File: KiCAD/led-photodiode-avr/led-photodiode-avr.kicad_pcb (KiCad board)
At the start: 4 copper layers, 68.6 x 80 mm, 62 parts, among them J1 Screw_Terminal_01x02, J2 Conn_02x08_Odd_Even, J3 ISP, J4 Conn_01x06_Pin, Q1 TTC1949, Q2 TTC1949, Q3 TTC1949, Q4 TTC1949, U1 REF3040AIDBZT, U10 AZ1117CH2-5.0, U2 AZ1117CH2-5.0, U3 OPA365xxD, U5 DDC112, U6 LTC1380, U7 ATmega328-A, U8 OPA365xxD, U9 LTC2631, Y1 CO_16MHZ

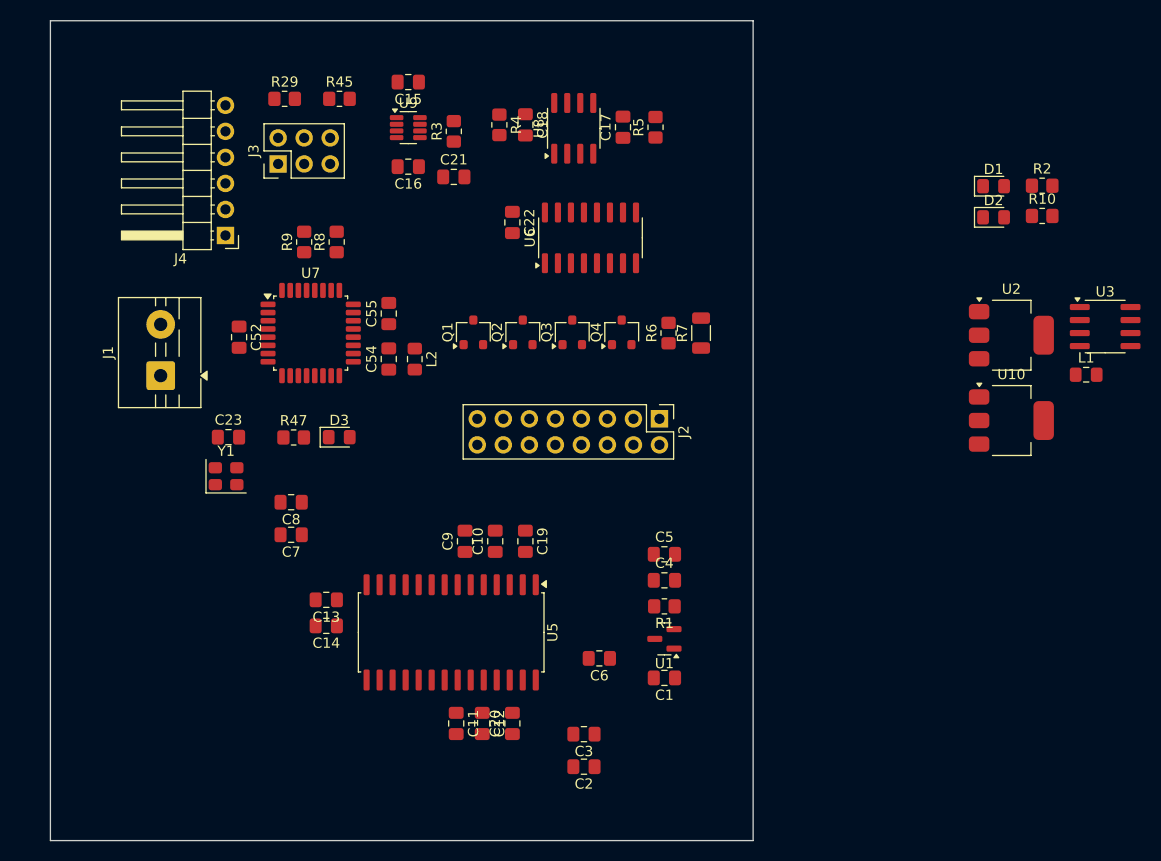
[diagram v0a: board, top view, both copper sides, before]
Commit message: routing done
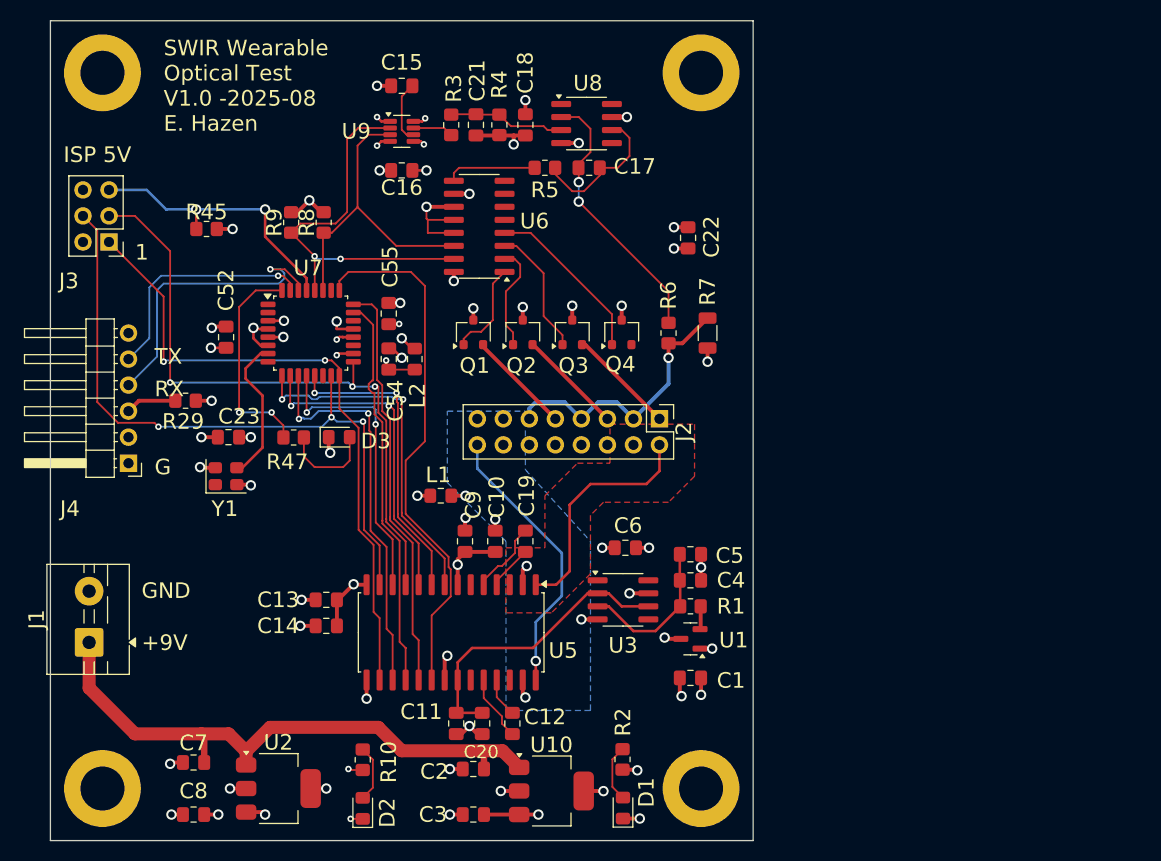
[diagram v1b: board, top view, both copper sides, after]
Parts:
- added H1: MountingHole, MountingHole:MountingHole_4.3mm_M4_DIN965_Pad, F.Cu at (121.9, 62.2)
- added H2: MountingHole, MountingHole:MountingHole_4.3mm_M4_DIN965_Pad, F.Cu at (180.3, 62.2)
- added H3: MountingHole, MountingHole:MountingHole_4.3mm_M4_DIN965_Pad, F.Cu at (121.9, 132.1)
- added H4: MountingHole, MountingHole:MountingHole_4.3mm_M4_DIN965_Pad, F.Cu at (180.3, 132.1)
- moved R10 84.9 mm to (147.3, 129.3), turned to 90 degrees
- moved D2 84.4 mm to (147.3, 134.0), turned to 90 degrees
- moved U2 84.1 mm to (139.1, 132.1)
- moved D1 70.6 mm to (172.7, 134.0), turned to 90 degrees
- moved R2 69.4 mm to (172.7, 129.2), turned to 90 degrees
- moved L1 64.1 mm to (154.9, 103.5)
- moved U10 57.6 mm to (165.7, 132.3)
- moved U3 54.1 mm to (172.7, 113.7)
- moved C8 31.9 mm to (130.8, 134.6)
- moved R29 31.0 mm to (130.0, 94.2), turned to 180 degrees
- moved J1 27.0 mm to (120.6, 117.8)
- moved C7 24.2 mm to (130.8, 129.5)
- moved J4 24.2 mm to (124.5, 100.3)
- moved J3 18.2 mm to (122.6, 78.7), turned to 180 degrees
- moved R45 18.2 mm to (132.1, 77.5)
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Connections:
- C16 pad 1: +5VA -> VCC
- D1 pad 1: GND -> Earth
- J2 pad 1: /LED_driver/LED_1 -> /LED_driver/LED_3
- J2 pad 9: /LED_driver/LED_3 -> /LED_driver/LED_1
- U6 pad 11: Earth -> GND
- U6 pad 12: Earth -> GND
- U6 pad 13: Earth -> GND
- U9 pad 5: +5VA -> VCC
- U9 pad 8: +5VA -> VCC
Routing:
- net /MOSI: track 0.00 -> 67.1 mm, vias 0 -> 3
- net /SCK: track 0.00 -> 63.7 mm, vias 0 -> 3
- net /MISO: track 0.00 -> 63.5 mm, vias 0 -> 2
- net VBUS: track 0.00 -> 57.6 mm
- net /PC2/ADC2: track 0.00 -> 52.0 mm
- net GND: track 0.00 -> 42.5 mm, vias 0 -> 23
- net Earth: track 0.00 -> 41.7 mm, vias 0 -> 22
- net /PC1/ADC1: track 0.00 -> 40.4 mm
- net /PC0/ADC0: track 0.00 -> 38.9 mm
- net /PD7: track 0.00 -> 38.5 mm, vias 0 -> 2
- net /SCL: track 0.00 -> 38.3 mm, vias 0 -> 2
- net /PD5: track 0.00 -> 34.7 mm, vias 0 -> 2
- net VCC: track 0.00 -> 32.3 mm, vias 0 -> 15
- net /PD6/OC0A: track 0.00 -> 31.5 mm, vias 0 -> 2
- net /SDA: track 0.00 -> 30.6 mm
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- added copper zone on In2.Cu, net +5VA
- added copper zone on B.Cu, net Earth
- added copper zone on F.Cu, net Earth
- added copper zone on In2.Cu, net VCC
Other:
- board text added: "+9V"
- board text added: "1"
- board text added: "G"
- board text added: "GND"
- board text added: "ISP 5V"
- board text added: "RX"
- board text added: "SWIR Wearable Optical Test V1.0 -2025-08 E. Hazen"
- board text added: "TX"
